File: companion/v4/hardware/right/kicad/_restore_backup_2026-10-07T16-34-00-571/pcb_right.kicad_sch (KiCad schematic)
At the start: 55 parts, among them J1 TF31-6S-0.5SH_800_, J2 speaker, J3 USB_C_Receptacle_USB2.0_14P, J4 Conn_01x24_MountingPin, SW1 SW_BOOT, SW3 SW_RESET, U2 MAX98357AETE_T, U3 USBLC6-2SC6, U4 ESP32-S3-MINI-1, U5 TLV75528PDBV, U6 TPS63001, U7 TLV75515PDBV

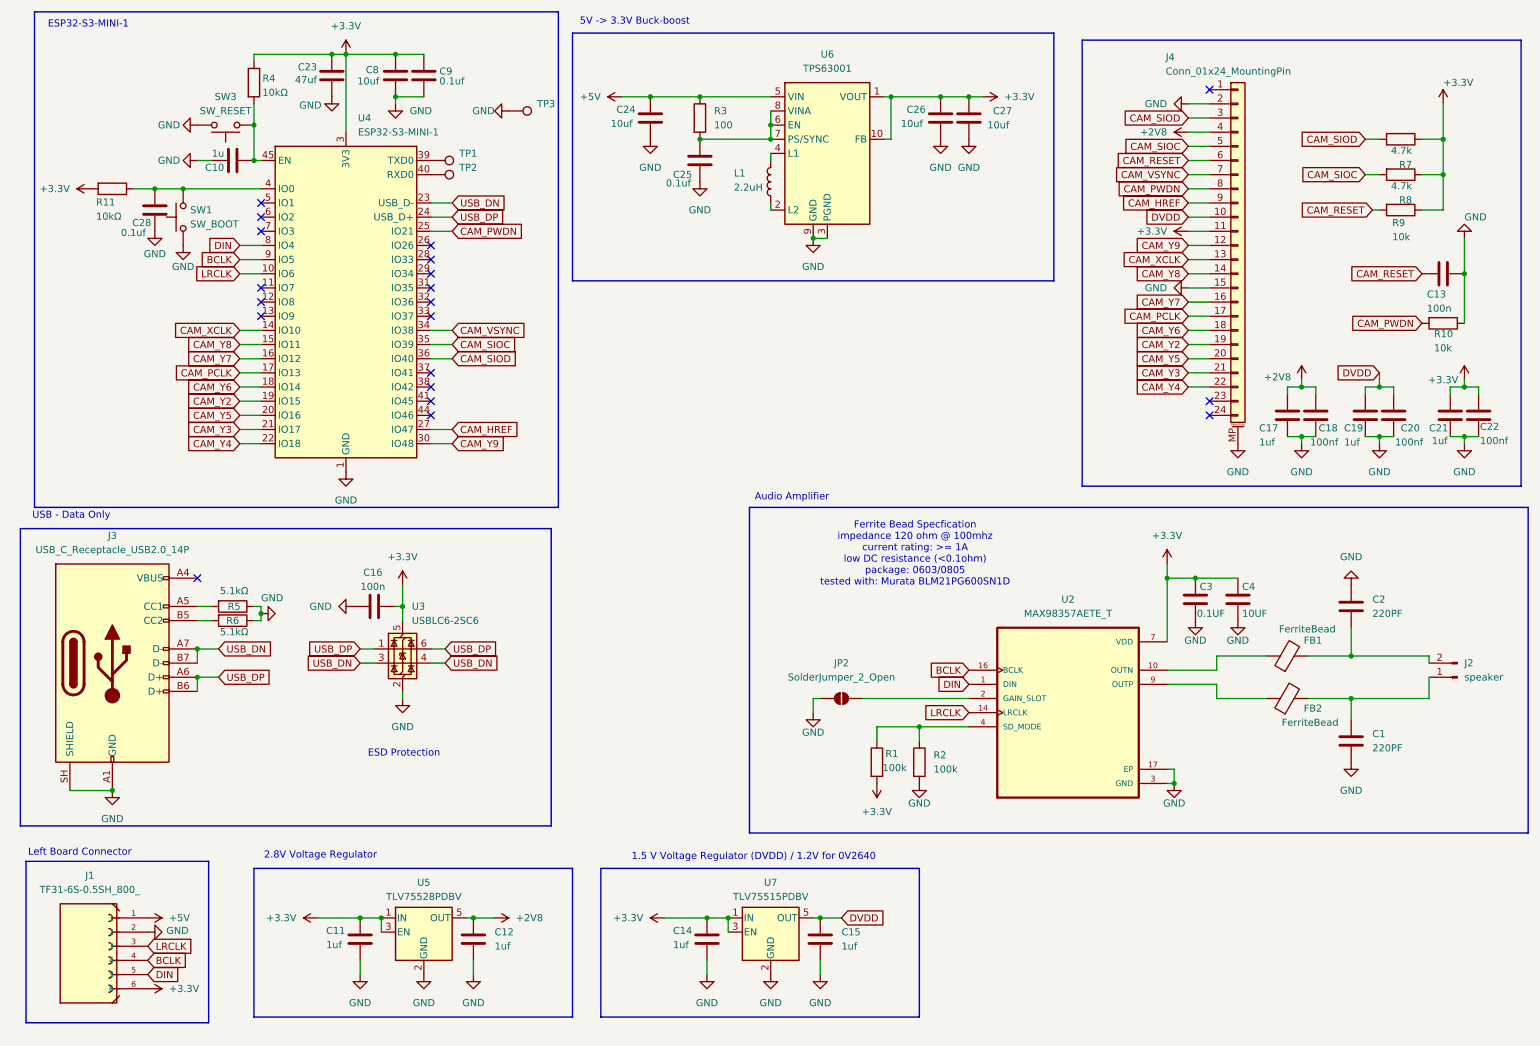
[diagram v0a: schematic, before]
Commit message: rev 2 - mcu changes and other various fixes
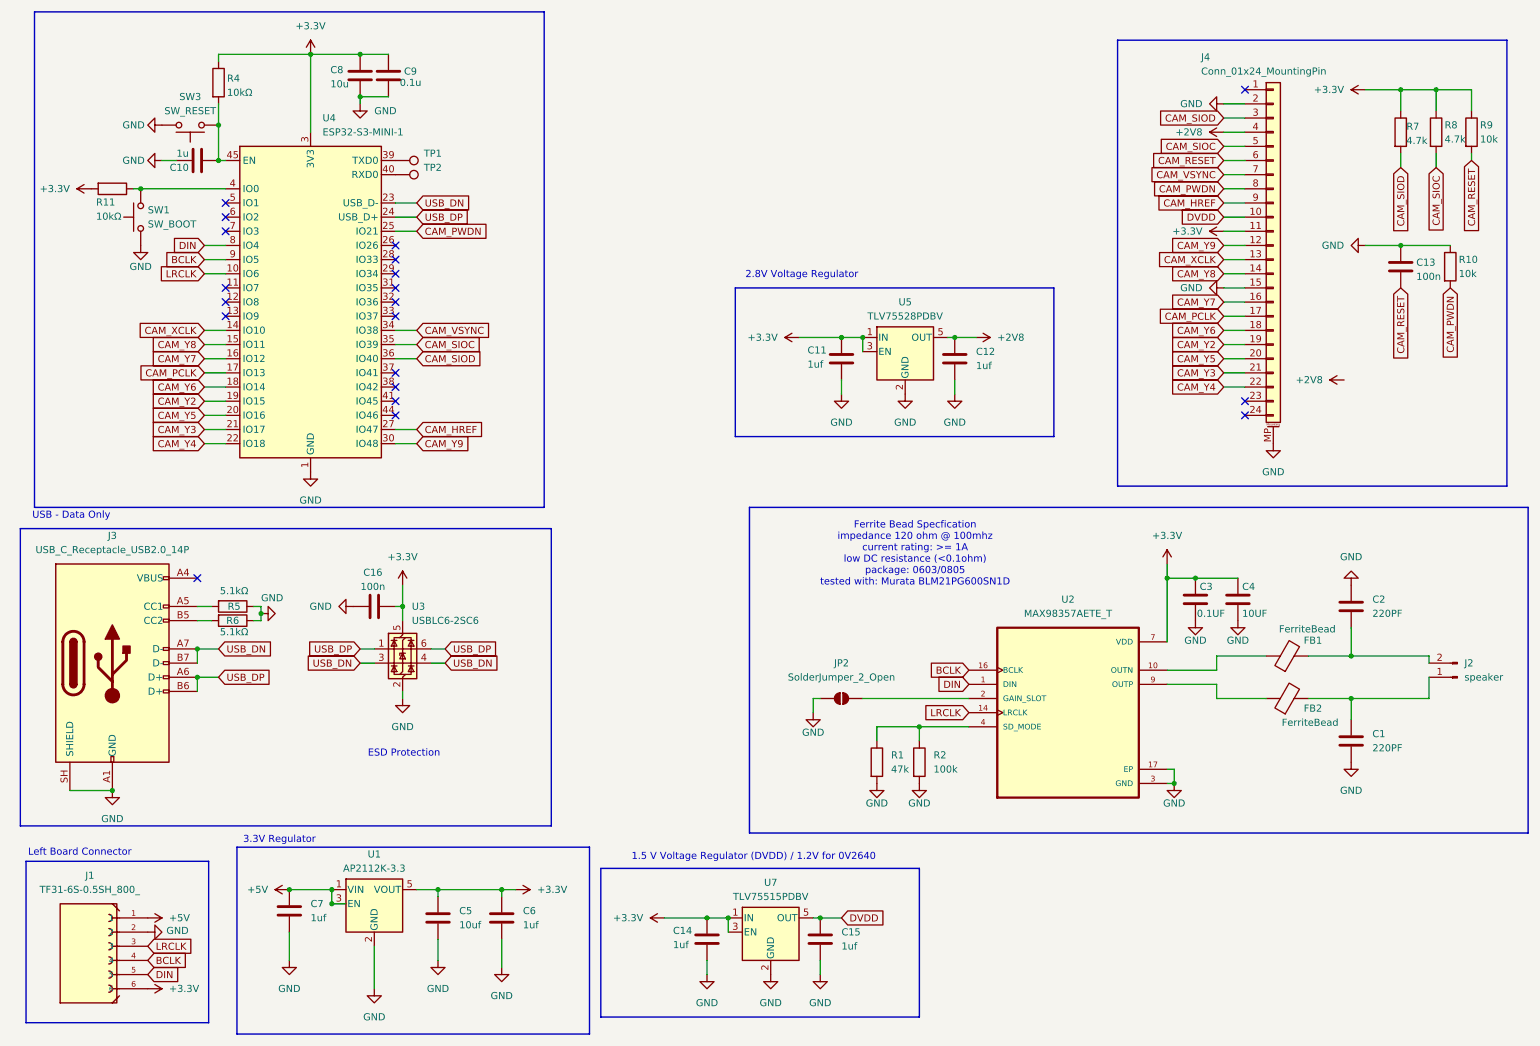
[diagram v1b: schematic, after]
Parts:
- removed C17, C19, C21: 1uf, symbol Device:C
- removed C18, C20, C22: 100nf, symbol Device:C
- removed C23: 47uf, symbol Device:C
- removed C24, C26, C27: 10uf, symbol Device:C
- removed C25, C28: 0.1uf, symbol Device:C
- removed L1: 2.2uH, Package_SON:Texas_DRC0010J_ThermalVias, symbol Device:L
- removed R3: 100, Resistor_SMD:R_0805_2012Metric_Pad1.20x1.40mm_HandSolder, symbol Device:R
- removed TP3: GND, symbol Connector:TestPoint
- removed U6: TPS63001, Package_SON:Texas_DRC0010J_ThermalVias, symbol Regulator_Switching:TPS63001
- added C5: 10uf, symbol Device:C
- added C6, C7: 1uf, symbol Device:C
- added U1: AP2112K-3.3, Package_TO_SOT_SMD:SOT-23-5, symbol Regulator_Linear:AP2112K-3.3
- C8: value 10uf -> 10u
- C9: value 0.1uf -> 0.1u
- R1: value 100k -> 47k
- TP1: value TX -> TestPoint
- TP2: value RX -> TestPoint
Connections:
- net +3.3V: now also C5.1, C6.1, U1.5 (VOUT); no longer R1.2
- net +5V: now also C7.1, U1.1 (VIN), U1.3 (EN)
- net GND: now also R1.2, C5.2, C6.2, C7.2, U1.2 (GND)
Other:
- note added: "3.3V Regulator"
- note removed: "5V -> 3.3V Buck-boost"
- note removed: "Audio Amplifier"
- note removed: "ESP32-S3-MINI-1"
- moved on the sheet: C10, C11, C12, C13, C8, C9, J4, R10, R4, R7, R8, R9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
